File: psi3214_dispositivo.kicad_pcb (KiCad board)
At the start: 2 copper layers, 43 x 44 mm, 20 parts, among them J1 Screw_Terminal_01x02, J2 Screw_Terminal_01x03, J3 Conn_01x02_Socket, J4 Conn_01x03, J5 Conn_01x02_Socket, J6 Screw_Terminal_01x02, U1 TL072_sim

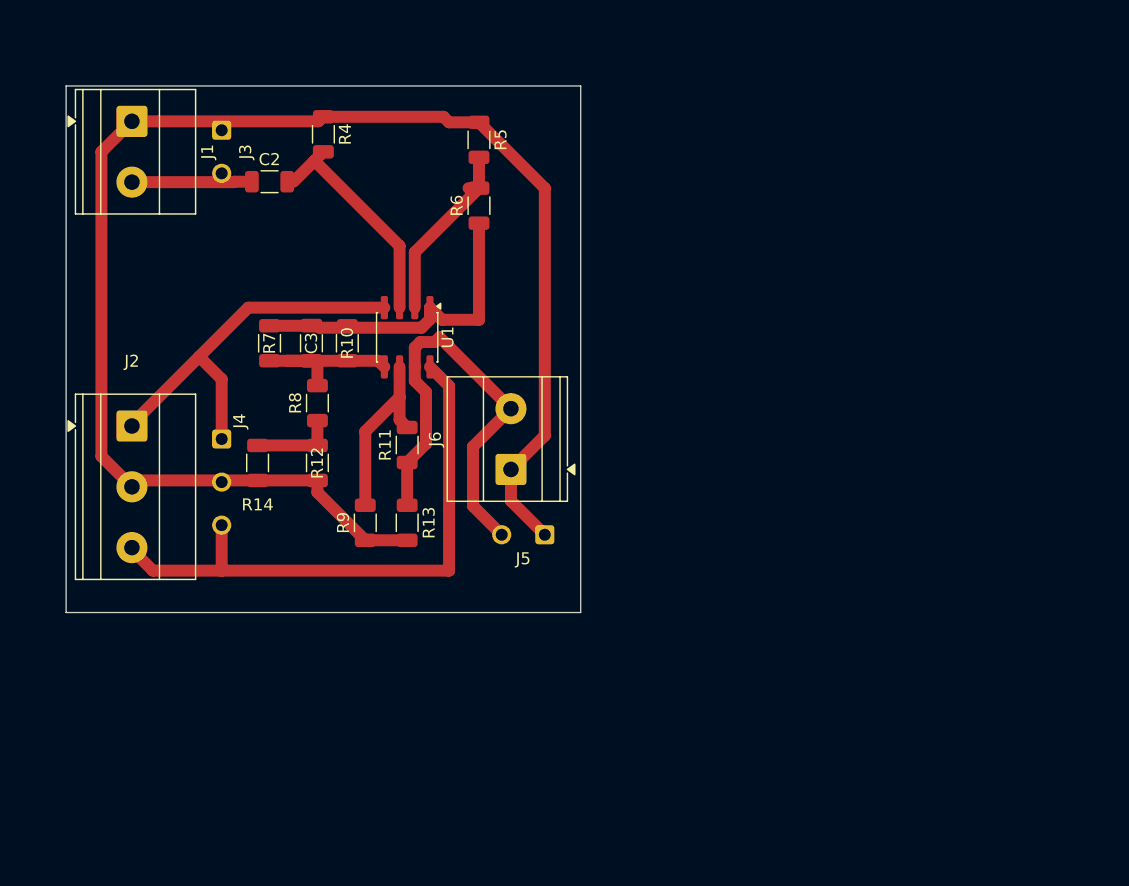
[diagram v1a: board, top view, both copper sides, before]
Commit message: Pot added
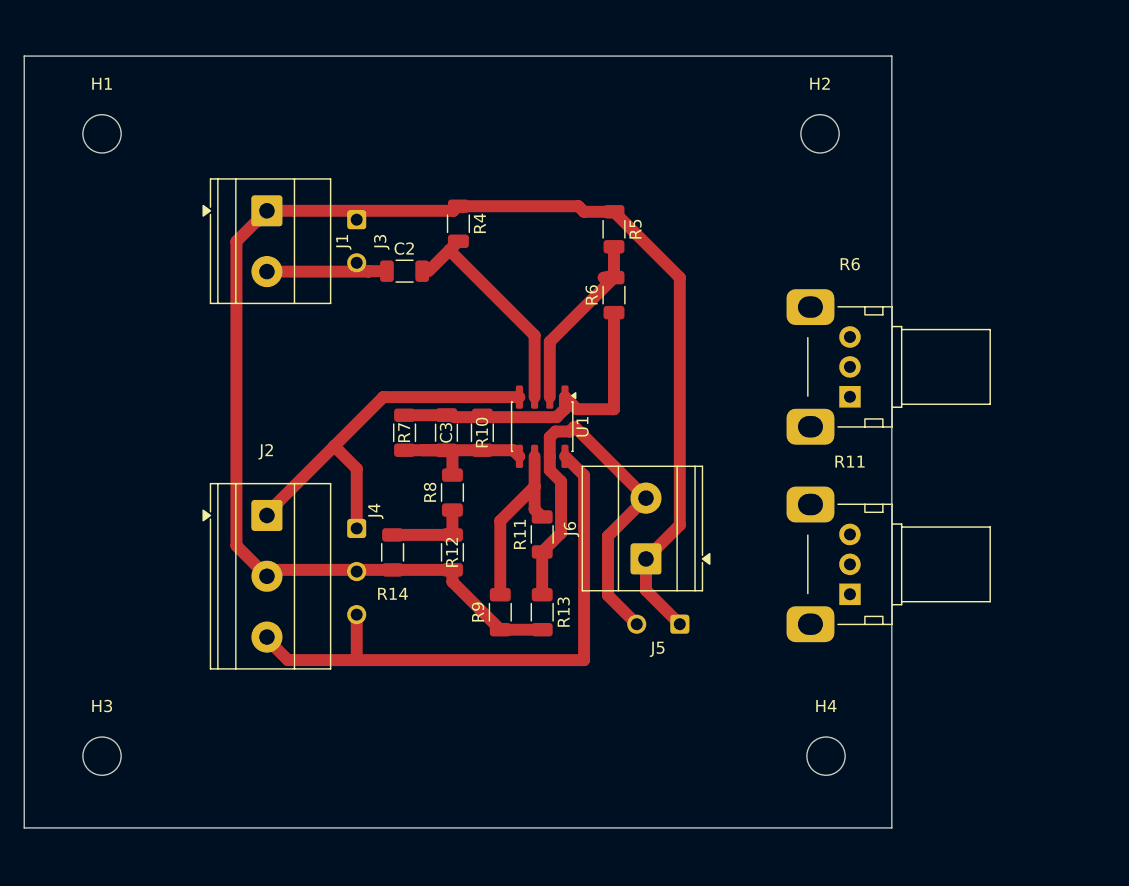
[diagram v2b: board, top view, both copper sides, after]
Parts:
- added H1: MountingHole, MountingHole:MountingHole_3.2mm_M3, F.Cu at (137.5, 43.0)
- added H2: MountingHole, MountingHole:MountingHole_3.2mm_M3, F.Cu at (197.5, 43.0)
- added H3: MountingHole, MountingHole:MountingHole_3.2mm_M3, F.Cu at (137.5, 95.0)
- added H4: MountingHole, MountingHole:MountingHole_3.2mm_M3, F.Cu at (198.0, 95.0)
- added R11: Potentiometer, Potentiometer_THT:Potentiometer_Alps_RK09K_Single_Horizontal, F.Cu at (200.0, 81.5)
- added R6: Potentiometer, Potentiometer_THT:Potentiometer_Alps_RK09K_Single_Horizontal, F.Cu at (200.0, 65.0)
- moved C2 13.5 mm to (162.8, 54.5)
- moved J1 13.5 mm to (151.3, 49.4)
- moved R4 13.5 mm to (167.3, 50.5)
- moved R5 13.5 mm to (180.3, 51.0)
- moved R6 13.5 mm to (180.3, 56.5)
- moved C3 13.5 mm to (166.3, 68.0)
- moved J2 13.5 mm to (151.3, 74.9)
- moved J3 13.5 mm to (158.8, 50.2)
- moved J4 13.5 mm to (158.8, 76.0)
- moved J5 13.5 mm to (185.8, 84.0)
- moved J6 13.5 mm to (183.0, 78.5)
- moved R10 13.5 mm to (169.3, 68.0)
- moved R11 13.5 mm to (174.3, 76.5)
- moved R12 13.5 mm to (166.8, 78.0)
- moved R13 13.5 mm to (174.3, 83.0)
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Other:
- board size 43 x 44 mm -> 72.5 x 64.5 mm

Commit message: Done
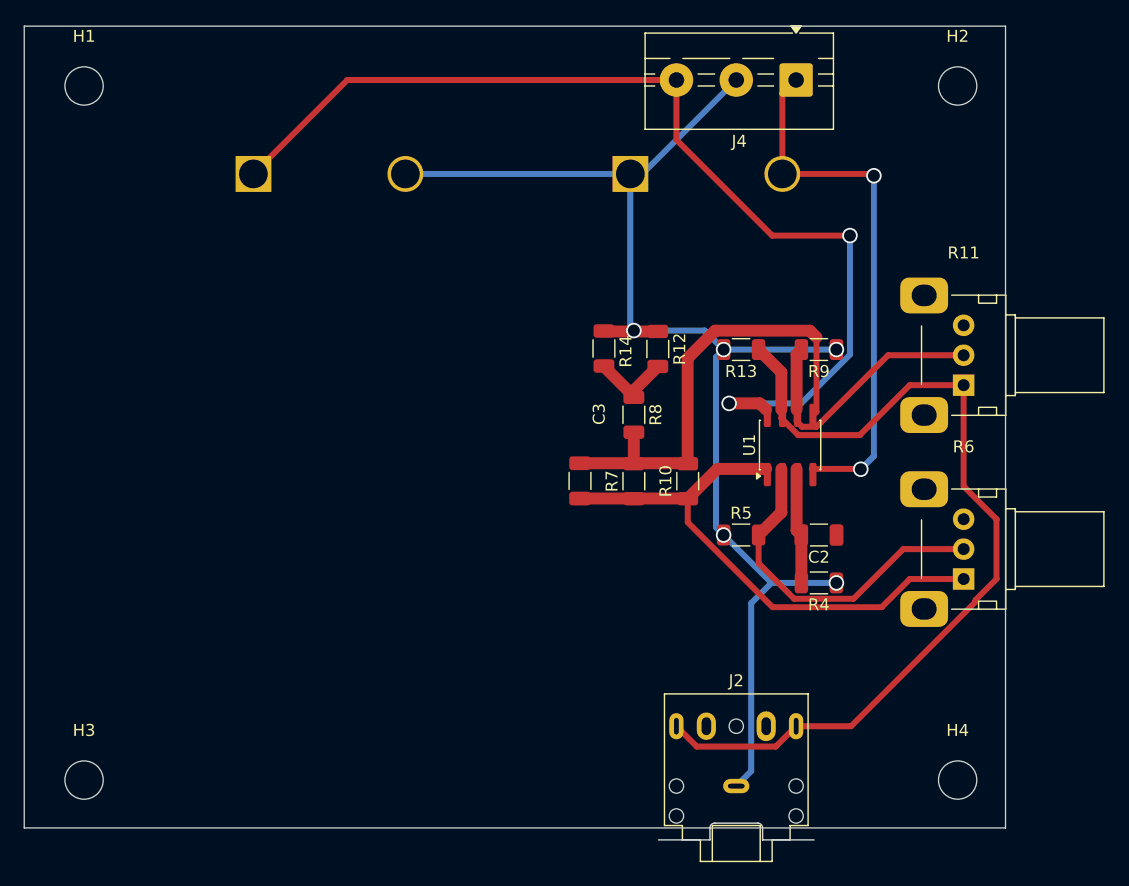
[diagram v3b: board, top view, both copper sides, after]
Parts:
- removed J1, J6: Screw_Terminal_01x02, TerminalBlock_Phoenix:TerminalBlock_Phoenix_MKDS-1,5-2-5.08_1x02_P5.08mm_Horizontal
- removed J3, J5: Conn_01x02_Socket, Connector_Wire:SolderWire-0.1sqmm_1x02_P3.6mm_D0.4mm_OD1mm
- removed the R11 at (174.3, 76.5)
- removed the R11 at (200.0, 81.5)
- removed the R6 at (200.0, 65.0)
- removed the R6 at (180.3, 56.5)
- added BT1: Battery, Beserrovsky:BatteryHolder_Eagle_12BH611-GR, B.Cu at (150.2, 46.4)
- added BT2: Battery, Beserrovsky:BatteryHolder_Eagle_12BH611-GR, B.Cu at (181.7, 46.4)
- added R11: Potentiometer, Potentiometer_THT:Potentiometer_Alps_RK09K_Single_Horizontal, F.Cu at (209.5, 64.0)
- added R6: Potentiometer, Potentiometer_THT:Potentiometer_Alps_RK09K_Single_Horizontal, F.Cu at (209.5, 80.2)
- J2: value Screw_Terminal_01x03 -> AudioJack3; footprint TerminalBlock_Phoenix:TerminalBlock_Phoenix_MKDS-1,5-3-5.08_1x03_P5.08mm_Horizontal -> Connector_Audio:Jack_3.5mm_CUI_SJ1-3525N_Horizontal
- J4: footprint Connector_Wire:SolderWire-0.1sqmm_1x03_P3.6mm_D0.4mm_OD1mm -> TerminalBlock:TerminalBlock_MaiXu_MX126-5.0-03P_1x03_P5.00mm
- moved J4 52.5 mm to (195.5, 38.5), turned to 180 degrees
- moved J2 45.3 mm to (190.5, 97.5), turned to 0 degrees
- moved R4 42.5 mm to (197.4, 80.5), turned to 180 degrees
- moved C2 41.0 mm to (197.4, 76.5), turned to 180 degrees
- moved R9 34.5 mm to (197.4, 61.0), turned to 180 degrees
- moved R5 27.7 mm to (190.9, 76.5), turned to 0 degrees
- moved R13 27.5 mm to (190.9, 61.0), turned to 180 degrees
- moved R14 24.5 mm to (179.4, 60.9), turned to -90 degrees
- moved R12 24.2 mm to (183.9, 61.0), turned to -90 degrees
- moved U1 20.8 mm to (195.0, 69.0), turned to 90 degrees
- moved R7 19.6 mm to (181.9, 72.0), turned to 90 degrees
- moved R10 17.6 mm to (186.4, 72.0), turned to 90 degrees
- moved R8 16.5 mm to (181.9, 66.5), turned to -90 degrees
- moved H2 12.2 mm to (209.0, 39.0)
- moved C3 11.9 mm to (177.4, 72.0), turned to 90 degrees
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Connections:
- net /saida_amp1 renamed saida_amp1
- net /saida_cap renamed saida_cap
- net /saida_filtro renamed saida_filtro
- C2 pad 1: /entrada -> entrada
- R13 pad 1: /saida -> saida
- U1 pad 7: /saida -> saida
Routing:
- net saida: track 0.00 -> 74.7 mm
- net /saida: track 37.9 -> 0.00 mm
- net +9V: track 48.9 -> 86.4 mm, vias 0 -> 2
- net saida_filtro: track 14.4 -> 39.8 mm
- net saida_amp1: track 27.3 -> 45.5 mm
- net GND: track 127.0 -> 111.5 mm, vias 0 -> 5
- net -9V: track 32.9 -> 46.1 mm, vias 0 -> 2
- net Net-(U1A--): track 15.7 -> 28.8 mm
- net /entrada: track 10.0 -> 0.00 mm
- net saida_cap: track 18.8 -> 9.69 mm
- net Net-(U1B--): track 15.5 -> 22.8 mm
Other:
- board size 72.5 x 64.5 mm -> 82 x 67 mm
